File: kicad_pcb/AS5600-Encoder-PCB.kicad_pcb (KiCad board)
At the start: 2 copper layers, 22.6 x 13.3 mm, 11 parts, among them IC1 AS5600-ASOM, J1 Conn_01x04_Male, J2 Conn_01x04_Male

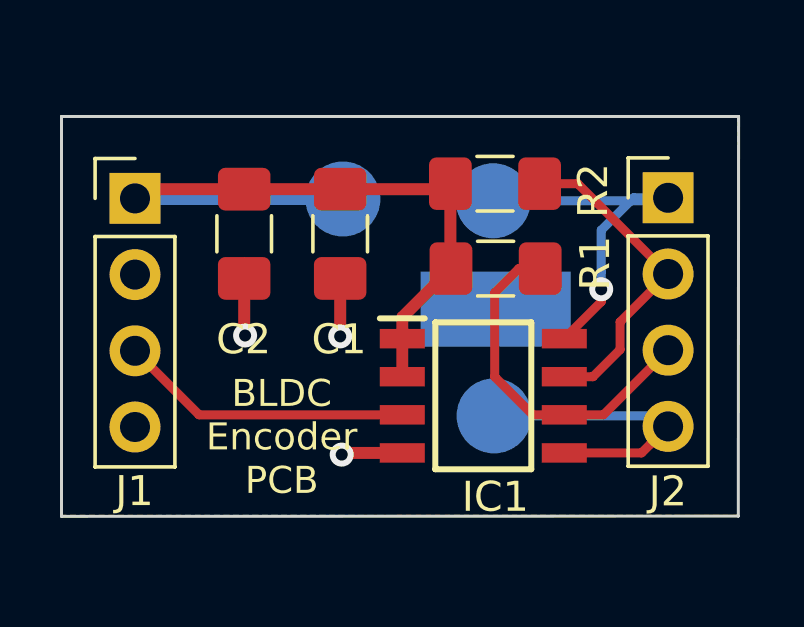
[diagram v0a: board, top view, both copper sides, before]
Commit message: Added holes, gerbers - SMD PCB
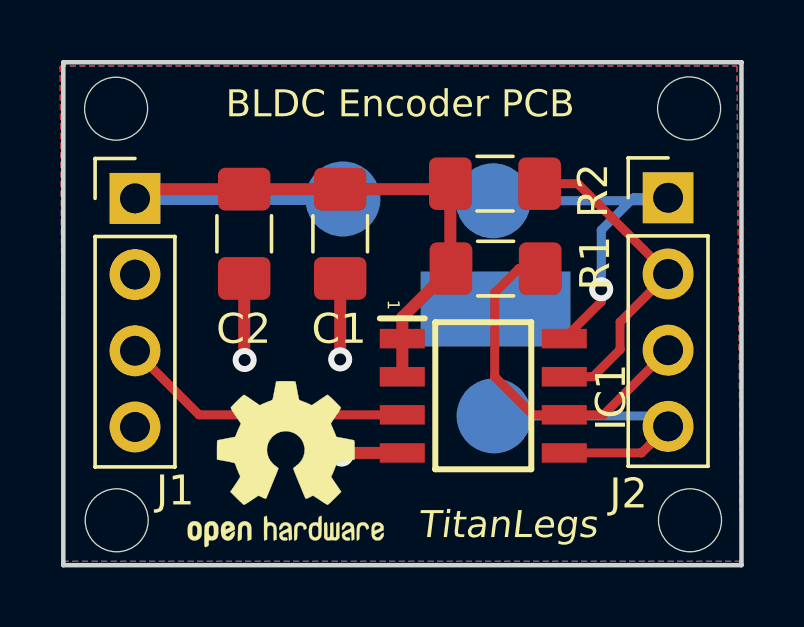
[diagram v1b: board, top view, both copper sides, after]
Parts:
- added REF**: OSHW-Logo2_7.3x6mm_SilkScreen, Symbol:OSHW-Logo2_7.3x6mm_SilkScreen, F.Cu at (197.9, 160.2)
- added REF**: MountingHole_2.1mm, MountingHole:MountingHole_2.1mm, F.Cu at (211.4, 148.3)
- added REF**: MountingHole_2.1mm, MountingHole:MountingHole_2.1mm, F.Cu at (192.3, 148.4)
- added REF**: MountingHole_2.1mm, MountingHole:MountingHole_2.1mm, F.Cu at (211.4, 162.1)
- added |: MountingHole_2.1mm, MountingHole:MountingHole_2.1mm, F.Cu at (192.3, 162.1)
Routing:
- net GND: track 6.40 -> 7.98 mm
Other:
- board size 22.6 x 13.3 mm -> 22.6 x 16.8 mm
- board text added: "---> CLK"
- board text added: "--> CCLK"
- board text added: "1"
- board text added: "SRA-VJTI"
- board text added: "TitanLegs"
- board text removed: "SRA VJTI"
- board text removed: "______> CLK"
- board text removed: "_______> CCLK"
